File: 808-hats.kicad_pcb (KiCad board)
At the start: 2 copper layers, 155 parts, among them J1 ohfilt-10k, J10 noisepresel, J11 noisein-pre, J12 noiseoutsrc, J2 chfilt-10k, J3 ohfilten, J4 chfilten, J5 trig/accent, J6 output, J7 noisesel, J8 noisein, J9 noiseout, P1 MTA-156-4, Q1 BC546, Q10 BC546, Q11 BC546, Q12 BC546, Q13 BC546, Q14 BC546, Q2 BC546, Q3 BC556, Q4 BC556, Q5 BC546, Q6 BC546, Q7 BC546, Q8 BC546, Q9 BC546, U1 40106, U2 TL074, U3 78L05, U4 TL072

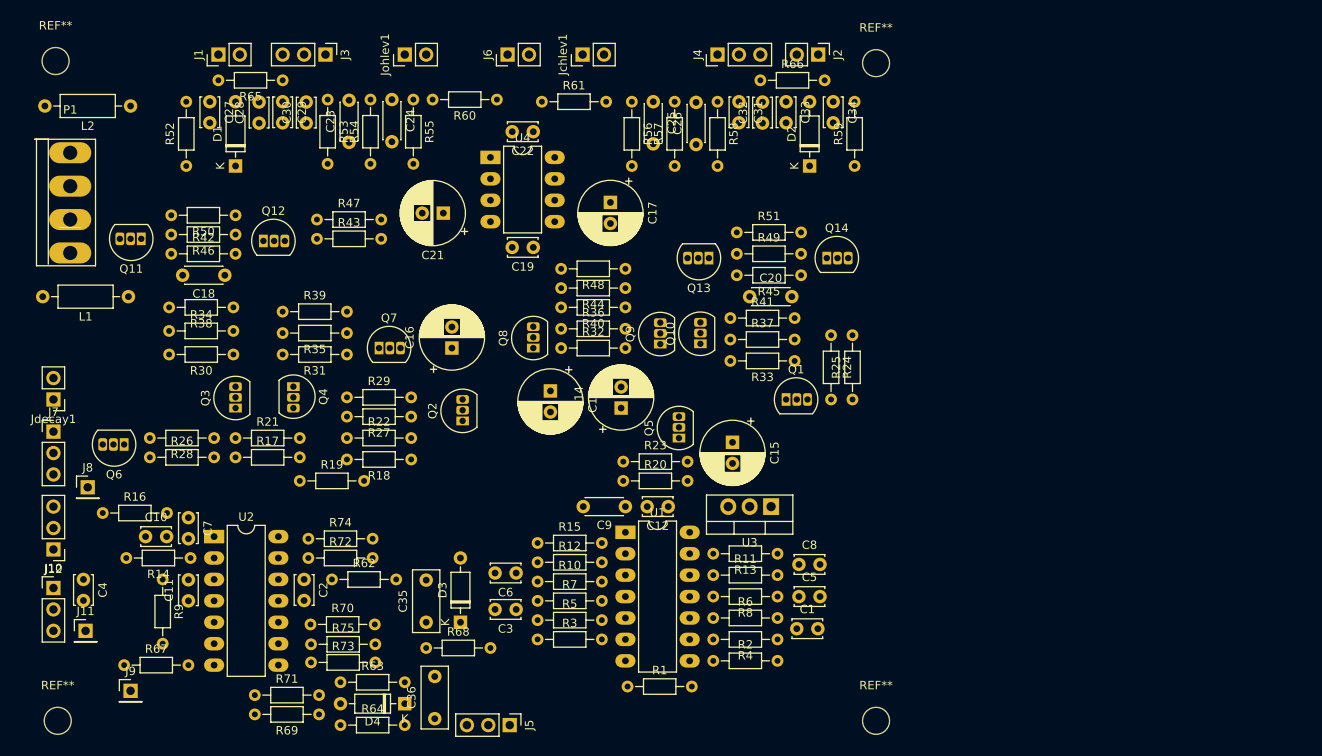
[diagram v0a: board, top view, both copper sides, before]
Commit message: much layout work
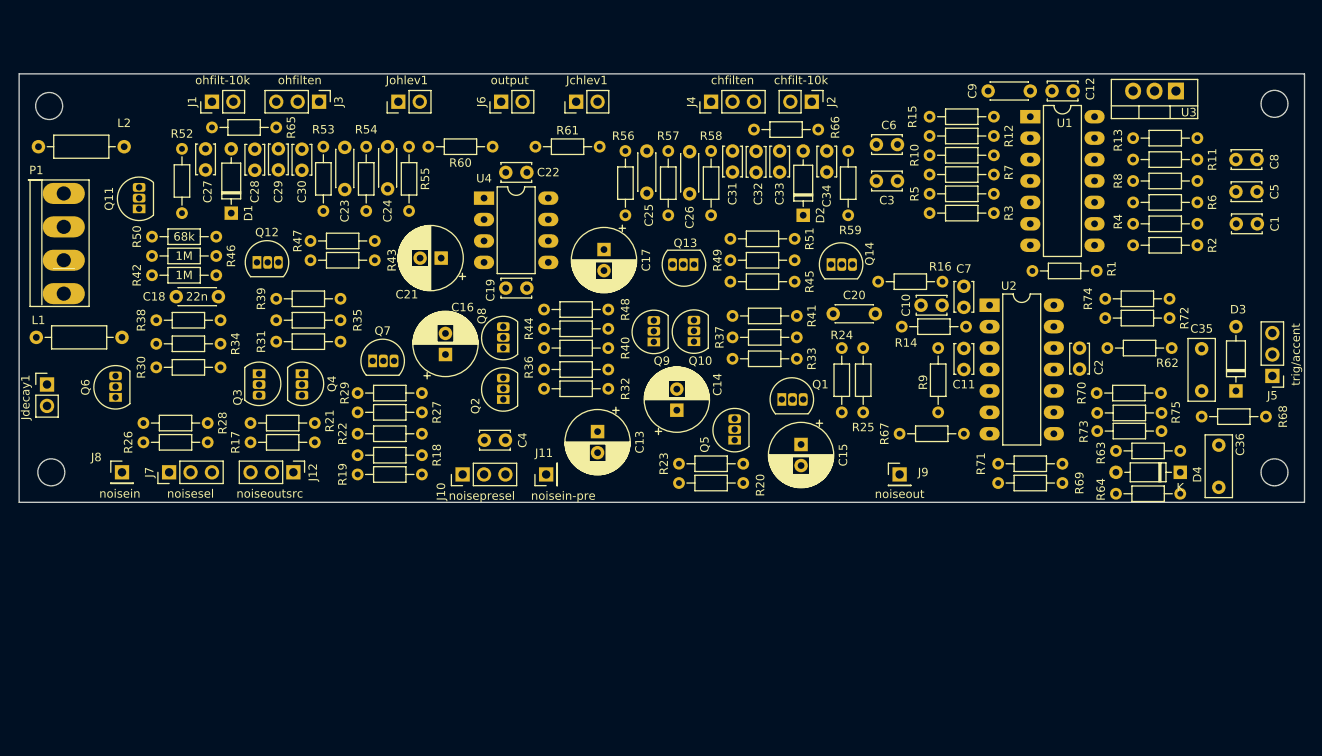
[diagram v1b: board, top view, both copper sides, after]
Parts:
- moved J5 99.5 mm to (205.7, 86.6), turned to 180 degrees
- moved R72 98.7 mm to (185.9, 79.8)
- moved R74 98.7 mm to (185.9, 77.5)
- moved R70 97.2 mm to (184.9, 88.6)
- moved R73 97.2 mm to (185.0, 93.2)
- moved R75 97.2 mm to (185.0, 91.0)
- moved C36 96.9 mm to (199.4, 99.8)
- moved C10 96.0 mm to (164.1, 78.2)
- moved C35 96.0 mm to (197.4, 88.4)
- moved D4 96.0 mm to (194.8, 98.0)
- moved R63 96.0 mm to (187.2, 95.5)
- moved R67 96.0 mm to (161.5, 93.5)
- moved R68 96.0 mm to (197.4, 91.4)
- moved R9 96.0 mm to (166.1, 83.3)
- moved C11 96.0 mm to (169.2, 85.9)
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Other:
- board outline added: 152.4 x 50.8 mm
